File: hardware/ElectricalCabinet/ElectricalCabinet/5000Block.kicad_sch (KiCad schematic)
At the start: 0 parts

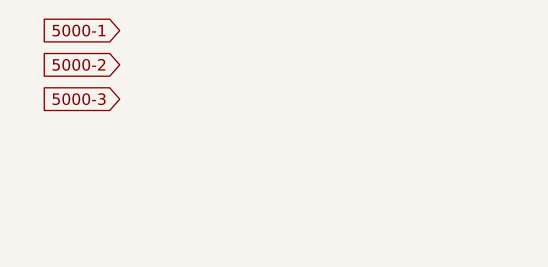
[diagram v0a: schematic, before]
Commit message: Electrical Cabinet done
Electrical Cabinet done, let me know if there are any changes or mistakes.
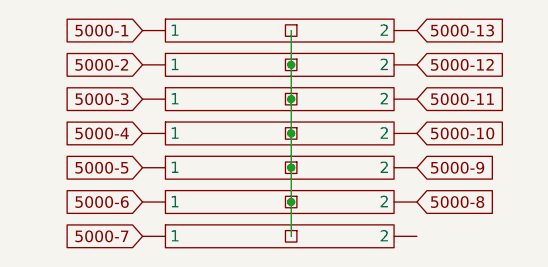
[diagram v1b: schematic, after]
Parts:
- added U77, U78, U79, U80, U81, U82, U83: (no value), symbol TrafficLightLibrary:Terminal_Block
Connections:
- net 5000-1: now also U77. (2)
- net 5000-2: now also U78. (2)
- net 5000-3: now also U79. (2)
- new net: U77. (2), U78. (2), U79. (2), U80. (2), U81. (2), U82. (2), U83. (2)
- new net 5000-10: U80. (2)
- new net 5000-11: U79. (2)
- new net 5000-12: U78. (2)
- new net 5000-13: U77. (2)
- new net 5000-4: U80. (2)
- new net 5000-5: U81. (2)
- new net 5000-6: U82. (2)
- new net 5000-7: U83. (2)
- new net 5000-8: U82. (2)
- new net 5000-9: U81. (2)
